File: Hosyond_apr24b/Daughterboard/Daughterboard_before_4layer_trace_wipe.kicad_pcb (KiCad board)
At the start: 4 copper layers, 155 x 80.6 mm, 150 parts, among them J1 USB-C 5V Sink, J30 J3P Hosyond +5V_SW solder pad, J31 J3A Hosyond UART_TX solder pad, J32 J3B Hosyond UART_RX solder pad, J33 J3C Hosyond I2C_SDA solder pad, J34 J3D Hosyond I2C_SCL solder pad, J35 J3E Hosyond GPIO2 solder pad, J36 J3F Hosyond GPIO3 solder pad, J37 J3G Hosyond GPIO14 solder pad, J38 J3H Hosyond GPIO21 solder pad, J39 J3I Hosyond GND solder pad, J4 UART JST-GH 1.25mm, J5 I2C male header 2.54mm, J6 Deep sleep pushbutton header, J7 2S balance input JST-XH, J8 Analog input header, J91 MCP23017 GPA0 solder pad, J910 MCP23017 GPB1 solder pad, J911 MCP23017 GPB2 solder pad, J912 MCP23017 GPB3 solder pad, J913 MCP23017 GPB4 solder pad, J914 MCP23017 GPB5 solder pad, J915 MCP23017 GPB6 solder pad, J916 MCP23017 GPB7 solder pad, J92 MCP23017 GPA1 solder pad, J925 MCP23017 INTA solder pad, J926 MCP23017 INTB solder pad, J927 MCP23017 RESET solder pad, J928 MCP23017 +3V3_SW solder pad, J929 MCP23017 GND solder pad, J93 MCP23017 GPA2 solder pad, J94 MCP23017 GPA3 solder pad, J95 MCP23017 GPA4 solder pad, J96 MCP23017 GPA5 solder pad, J97 MCP23017 GPA6 solder pad, J98 MCP23017 GPA7 solder pad, J99 MCP23017 GPB0 solder pad, Q1 CSD83325L, SW1 Pololu #2808 5V switch, SW2 Pololu #2808 3V3 switch, U1 BQ25887RGE 2S charger, U2 S-8252AAH-M6T1U, U3 AP63200WU 5V Buck, U4 AP63200WU 3V3 Buck, U5 ADS1115IDGS 0x48, U6 ADS1115IDGS 0x49, U7 MCP23017-E/SO

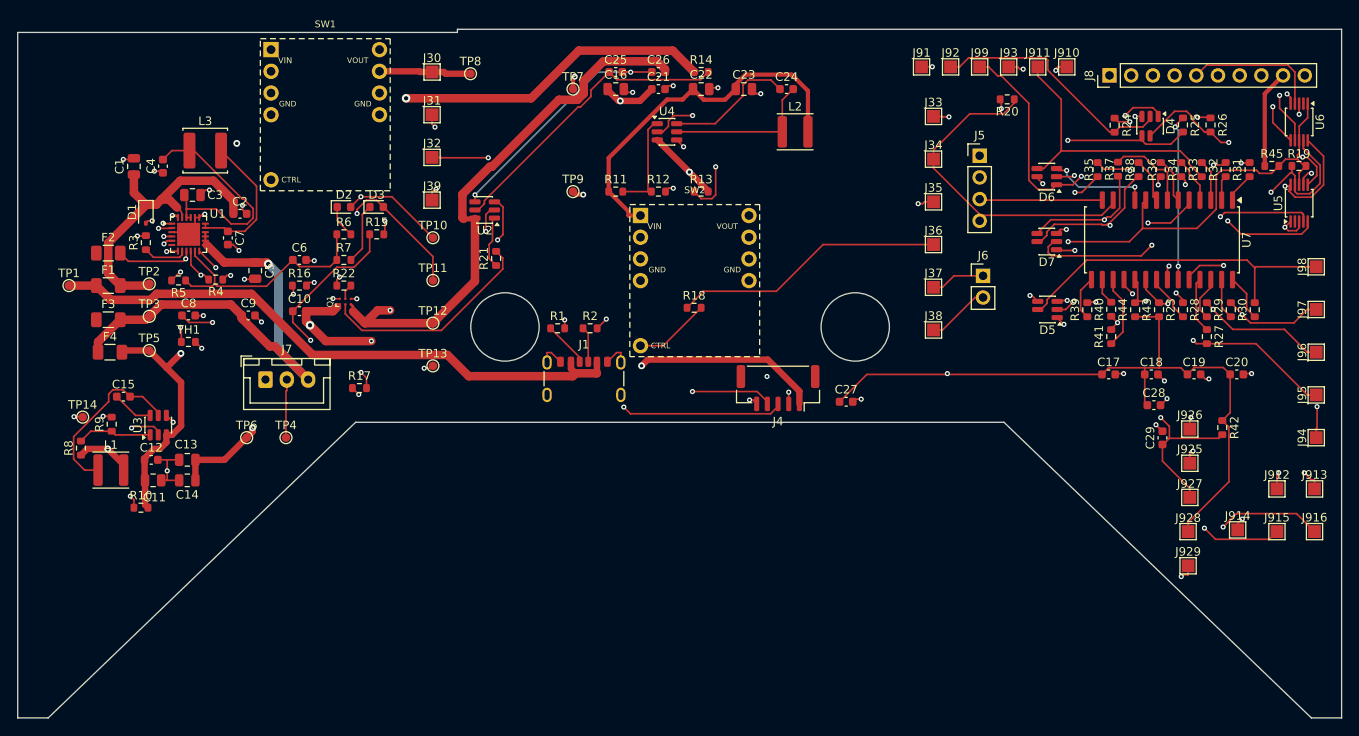
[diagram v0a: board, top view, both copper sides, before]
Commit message: k
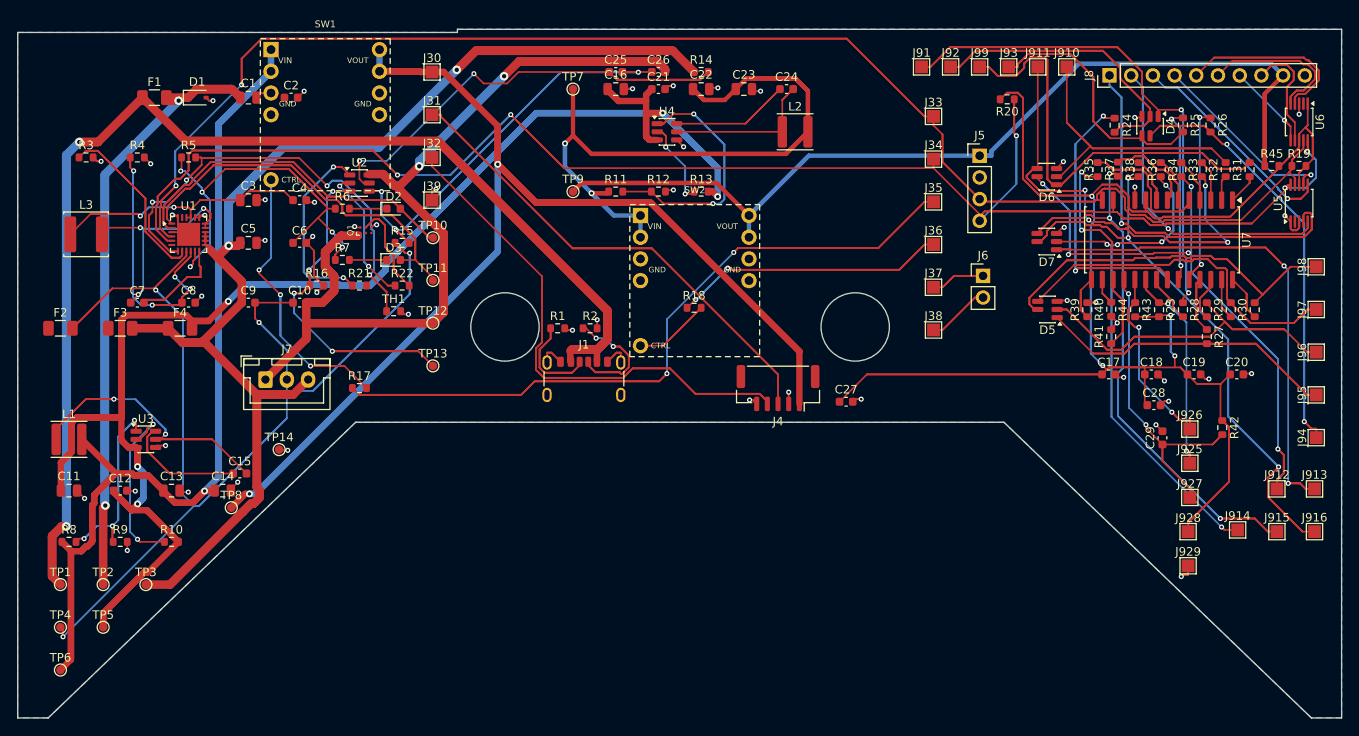
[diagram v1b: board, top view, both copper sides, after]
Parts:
- C8: value 100nF 10V X7R DNP -> 100nF 10V X7R
- D4, D5, D6, D7: value SP0504BAHTG 4ch GPIO TVS -> 4ch 3.3V GPIO TVS array TBD
- R3: value 806R 1% ILIM -> 806R 1% TBD
- R4: value 220R 1% CBSET -> TBD 1%
- moved TP8 58.0 mm to (35.0, 66.0)
- moved TP2 35.6 mm to (20.0, 75.0)
- moved TP1 35.0 mm to (15.0, 75.0)
- moved TP6 34.9 mm to (15.0, 85.0)
- moved TP4 34.5 mm to (15.0, 80.0)
- moved TP5 32.8 mm to (20.0, 80.0)
- moved TP3 31.4 mm to (25.0, 75.0)
- moved TH1 24.3 mm to (54.0, 43.0)
- moved TP14 23.3 mm to (40.6, 59.2)
- moved F1 22.7 mm to (26.0, 18.0)
- moved L3 17.0 mm to (18.0, 34.0)
- moved R4 17.0 mm to (24.0, 25.0)
- moved C4 16.5 mm to (43.0, 30.0), turned to 0 degrees
- moved C15 16.3 mm to (36.0, 62.0)
- moved R21 16.3 mm to (50.0, 40.0), turned to 0 degrees
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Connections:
- R4 pad 2: CELL_MID -> GND
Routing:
- net USB_VBUS: track 69.8 -> 257.3 mm, vias 0 -> 2
- net BAT_SYS: track 129.9 -> 299.8 mm, vias 4 -> 5
- net CELL_MID: track 62.0 -> 210.6 mm
- net +5V_SW: track 83.2 -> 226.0 mm, vias 1 -> 2
- net I2C_SDA: track 178.9 -> 319.4 mm, vias 3 -> 2
- net +3V3_SW_LOGIC: track 173.2 -> 301.3 mm, vias 3 -> 4
- net +5V: track 80.7 -> 189.0 mm, vias 2 -> 1
- net I2C_SCL: track 186.6 -> 287.6 mm, vias 2 -> 5
- net PACK_P: track 135.7 -> 232.3 mm
- net TS: track 14.1 -> 95.7 mm, vias 3 -> 4
- net CHG_IN: track 35.6 -> 116.6 mm, vias 0 -> 2
- net +3V3_SW: track 108.4 -> 181.8 mm, vias 1 -> 0
- net GPIO2: track 79.2 -> 149.6 mm, vias 3 -> 2
- net BATT_RAW_N: track 91.9 -> 152.1 mm, vias 3 -> 2
- net +3V3: track 66.9 -> 126.7 mm, vias 1 -> 2
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- added copper zone on B.Cu, net GND
- removed copper zone on In1.Cu, net GND
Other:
- copper layers 4 -> 2
